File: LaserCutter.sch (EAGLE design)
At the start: 126 parts, among them IC1 ATMEGA8U2, IC10 LM393D, IC11 74AHC1G02DBV, IC12 74AHC1G02DBV, IC13 74AHC1G08DBV, IC14 MAX6675, IC2 BEE module, IC3 MC34063, IC4 74AHC1G02DBV, IC5 74AHC1G08DBV, IC6 ATMEGA2560-16AU, IC7 CD4050D, IC8 LD1117S33, IC9 OPA340N, J1 X Stepper, J10 24V in, J11 Interface, J12 I2C, J13 SDMMC18650, J14 ISP, J15 UART3, J16 X Home, J17 Z Home, J18 Y Home, J19 Interlocks, J2 Reset En, J20 Spare, J21 Omega PCC-SMP-V-K, J3 USB, J4 Y Stepper, J5 Ground, J6 ISP, J7 Z Stepper, J8 Stepper disable, J9 Laser HV PSU, Q1 16 MHz, Q2 16MHz

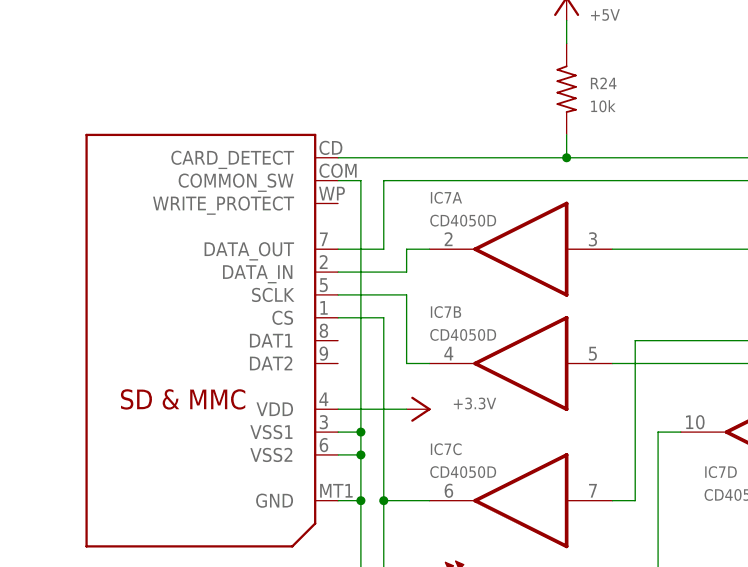
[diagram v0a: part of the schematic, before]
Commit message: a few tweaks
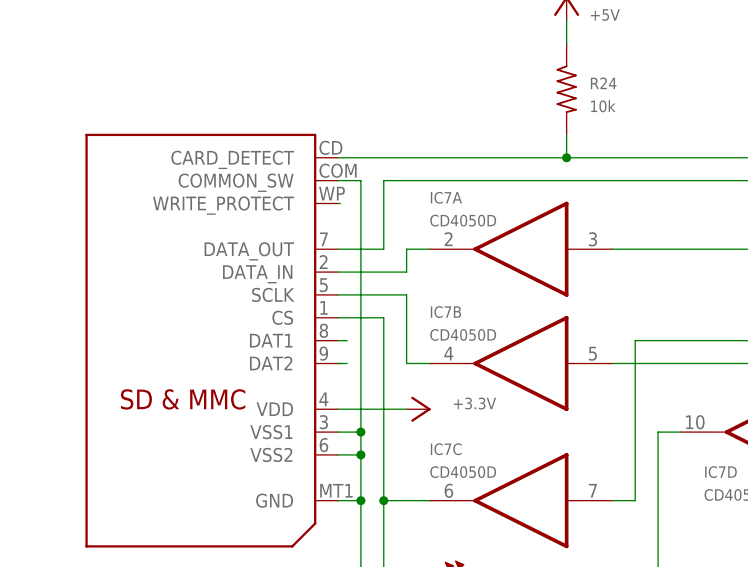
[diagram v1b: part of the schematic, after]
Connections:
- new net DAT1: J13.DAT1
- new net DAT2: J13.DAT2
- new net WP: J13.WRITE_PROTECT
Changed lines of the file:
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@@
 <setting verticaltext="up"/>
 </settings>
-<grid distance="0.1" unitdist="inch" unit="inch" style="lines" multiple="1" display="yes" altdistance="0.01" altunitdist="inch" altunit="inch"/>
+<grid distance="0.1" unitdist="inch" unit="inch" style="lines" multiple="1" display="no" altdistance="0.01" altunitdist="inch" altunit="inch"/>
 <layers>
-<layer number="1" name="Top" color="4" fill="1" visible="yes" active="no"/>
-<layer number="2" name="Route2" color="1" fill="3" visible="yes" active="no"/>
-<layer number="3" name="Route3" color="4" fill="3" visible="yes" active="no"/>
-<layer number="4" name="Route4" color="1" fill="4" visible="yes" active="no"/>
-<layer number="5" name="Route5" color="4" fill="4" visible="yes" active="no"/>
-<layer number="6" name="Route6" color="1" fill="8" visible="yes" active="no"/>
-<layer number="7" name="Route7" color="4" fill="8" visible="yes" active="no"/>
-<layer number="8" name="Route8" color="1" fill="2" visible="yes" active="no"/>
-<layer number="9" name="Route9" color="4" fill="2" visible="yes" active="no"/>
-<layer number="10" name="Route10" color="1" fill="7" visible="yes" active="no"/>
-<layer number="11" name="Route11" color="4" fill="7" visible="yes" active="no"/>
-<layer number="12" name="Route12" color="1" fill="5" visible="yes" active="no"/>
-<layer number="13" name="Route13" color="4" fill="5" visible="yes" active="no"/>
-<layer number="14" name="Route14" color="1" fill="6" visible="yes" active="no"/>
-<layer number="15" name="Route15" color="4" fill="6" visible="yes" active="no"/>
-<layer number="16" name="Bottom" color="1" fill="1" visible="yes" active="no"/>
-<layer number="17" name="Pads" color="2" fill="1" visible="yes" active="no"/>
-<layer number="18" name="Vias" color="2" fill="1" visible="yes" active="no"/>
-<layer number="19" name="Unrouted" color="6" fill="1" visible="yes" active="no"/>
-<layer number="20" name="Dimension" color="15" fill="1" visible="yes" active="no"/>
-<layer number="21" name="tPlace" color="7" fill="1" visible="yes" active="no"/>
-<layer number="22" name="bPlace" color="7" fill="1" visible="yes" active="no"/>
-<layer number="23" name="tOrigins" color="15" fill="1" visible="yes" active="no"/>
-<layer number="24" name="bOrigins" color="15" fill="1" visible="yes" active="no"/>
-<layer number="25" name="tNames" color="7" fill="1" visible="yes" active="no"/>
-<layer number="26" name="bNames" color="7" fill="1" visible="yes" active="no"/>
-<layer number="27" name="tValues" color="7" fill="1" visible="yes" active="no"/>
-<layer number="28" name="bValues" color="7" fill="1" visible="yes" active="no"/>
+<layer number="1" name="Top" color="4" fill="1" visible="no" active="no"/>
+<layer number="2" name="Route2" color="1" fill="3" visible="no" active="no"/>
+<layer number="3" name="Route3" color="4" fill="3" visible="no" active="no"/>
+<layer number="4" name="Route4" color="1" fill="4" visible="no" active="no"/>
+<layer number="5" name="Route5" color="4" fill="4" visible="no" active="no"/>
+<layer number="6" name="Route6" color="1" fill="8" visible="no" active="no"/>
+<layer number="7" name="Route7" color="4" fill="8" visible="no" active="no"/>
+<layer number="8" name="Route8" color="1" fill="2" visible="no" active="no"/>
+<layer number="9" name="Route9" color="4" fill="2" visible="no" active="no"/>
+<layer number="10" name="Route10" color="1" fill="7" visible="no" active="no"/>
+<layer number="11" name="Route11" color="4" fill="7" visible="no" active="no"/>
+<layer number="12" name="Route12" color="1" fill="5" visible="no" active="no"/>
+<layer number="13" name="Route13" color="4" fill="5" visible="no" active="no"/>
+<layer number="14" name="Route14" color="1" fill="6" visible="no" active="no"/>
+<layer number="15" name="Route15" color="4" fill="6" visible="no" active="no"/>
+<layer number="16" name="Bottom" color="1" fill="1" visible="no" active="no"/>
+<layer number="17" name="Pads" color="2" fill="1" visible="no" active="no"/>
+<layer number="18" name="Vias" color="2" fill="1" visible="no" active="no"/>
+<layer number="19" name="Unrouted" color="6" fill="1" visible="no" active="no"/>
+<layer number="20" name="Dimension" color="15" fill="1" visible="no" active="no"/>
+<layer number="21" name="tPlace" color="7" fill="1" visible="no" active="no"/>
+<layer number="22" name="bPlace" color="7" fill="1" visible="no" active="no"/>
+<layer number="23" name="tOrigins" color="15" fill="1" visible="no" active="no"/>
+<layer number="24" name="bOrigins" color="15" fill="1" visible="no" active="no"/>
+<layer number="25" name="tNames" color="7" fill="1" visible="no" active="no"/>
+<layer number="26" name="bNames" color="7" fill="1" visible="no" active="no"/>
+<layer number="27" name="tValues" color="7" fill="1" visible="no" active="no"/>
+<layer number="28" name="bValues" color="7" fill="1" visible="no" active="no"/>
 <layer number="29" name="tStop" color="7" fill="3" visible="no" active="no"/>
 <layer number="30" name="bStop" color="7" fill="6" visible="no" active="no"/>
@@
 <layer number="35" name="tGlue" color="7" fill="4" visible="no" active="no"/>
 <layer number="36" name="bGlue" color="7" fill="5" visible="no" active="no"/>
-<layer number="37" name="tTest" color="7" fill="1" visible="yes" active="no"/>
-<layer number="38" name="bTest" color="7" fill="1" visible="yes" active="no"/>
+<layer number="37" name="tTest" color="7" fill="1" visible="no" active="no"/>
+<layer number="38" name="bTest" color="7" fill="1" visible="no" active="no"/>
 <layer number="39" name="tKeepout" color="4" fill="11" visible="no" active="no"/>
 <layer number="40" name="bKeepout" color="1" fill="11" visible="no" active="no"/>
@@
 <layer number="44" name="Drills" color="7" fill="1" visible="no" active="no"/>
 <layer number="45" name="Holes" color="7" fill="1" visible="no" active="no"/>
-<layer number="46" name="Milling" color="3" fill="1" visible="yes" active="no"/>
-<layer number="47" name="Measures" color="7" fill="1" visible="yes" active="no"/>
-<layer number="48" name="Document" color="7" fill="1" visible="yes" active="no"/>
-<layer number="49" name="Reference" color="7" fill="1" visible="yes" active="no"/>
-<layer number="50" name="dxf" color="7" fill="1" visible="yes" active="no"/>
-<layer number="51" name="tDocu" color="7" fill="1" visible="yes" active="no"/>
-<layer number="52" name="bDocu" color="7" fill="1" visible="yes" active="no"/>
-<layer number="53" name="tGND_GNDA" color="7" fill="9" visible="yes" active="no"/>
-<layer number="54" name="bGND_GNDA" color="1" fill="9" visible="yes" active="no"/>
-<layer number="56" name="wert" color="7" fill="1" visible="yes" active="no"/>
-<layer number="60" name="p_dimension" color="6" fill="0" visible="yes" active="no"/>
-<layer number="61" name="pt_docu" color="7" fill="0" visible="yes" active="no"/>
+<layer number="46" name="Milling" color="3" fill="1" visible="no" active="no"/>
+<layer number="47" name="Measures" color="7" fill="1" visible="no" active="no"/>
+<layer number="48" name="Document" color="7" fill="1" visible="no" active="no"/>
+<layer number="49" name="Reference" color="7" fill="1" visible="no" active="no"/>
+<layer number="50" name="dxf" color="7" fill="1" visible="no" active="no"/>
+<layer number="51" name="tDocu" color="7" fill="1" visible="no" active="no"/>
+<layer number="52" name="bDocu" color="7" fill="1" visible="no" active="no"/>
+<layer number="53" name="tGND_GNDA" color="7" fill="9" visible="no" active="no"/>
+<layer number="54" name="bGND_GNDA" color="1" fill="9" visible="no" active="no"/>
+<layer number="56" name="wert" color="7" fill="1" visible="no" active="no"/>
+<layer number="60" name="p_dimension" color="6" fill="0" visible="no" active="no"/>
+<layer number="61" name="pt_docu" color="7" fill="0" visible="no" active="no"/>
 <layer number="91" name="Nets" color="2" fill="1" visible="yes" active="yes"/>
 <layer number="92" name="Busses" color="1" fill="1" visible="yes" active="yes"/>
@@
 </segment>
 </net>
+<net name="DAT1" class="0">
+<segment>
+<pinref part="J13" gate="G$1" pin="DAT1"/>
+<wire x1="43.18" y1="246.38" x2="44.196" y2="246.38" width="0.1524" layer="91"/>
+</segment>
+</net>
+<net name="DAT2" class="0">
+<segment>
+<pinref part="J13" gate="G$1" pin="DAT2"/>
+<wire x1="43.434" y1="243.84" x2="43.18" y2="243.84" width="0.1524" layer="91"/>
+<wire x1="43.18" y1="243.84" x2="44.196" y2="243.84" width="0.1524" layer="91"/>
+</segment>
+</net>
+<net name="WP" class="0">
+<segment>
+<pinref part="J13" gate="G$1" pin="WRITE_PROTECT"/>
+<wire x1="43.18" y1="261.62" x2="43.434" y2="261.62" width="0.1524" layer="91"/>
+</segment>
+</net>
